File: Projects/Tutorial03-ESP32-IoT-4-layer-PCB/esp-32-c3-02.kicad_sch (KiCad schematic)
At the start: 30 parts, among them J3 GSD090012SEU, U3 ESP32-C3-WROOM-02-H4, U4 CP2102N-Axx-xQFN20, U5 USBLC6-2SC6, U6 W25Q32JVSSIQ

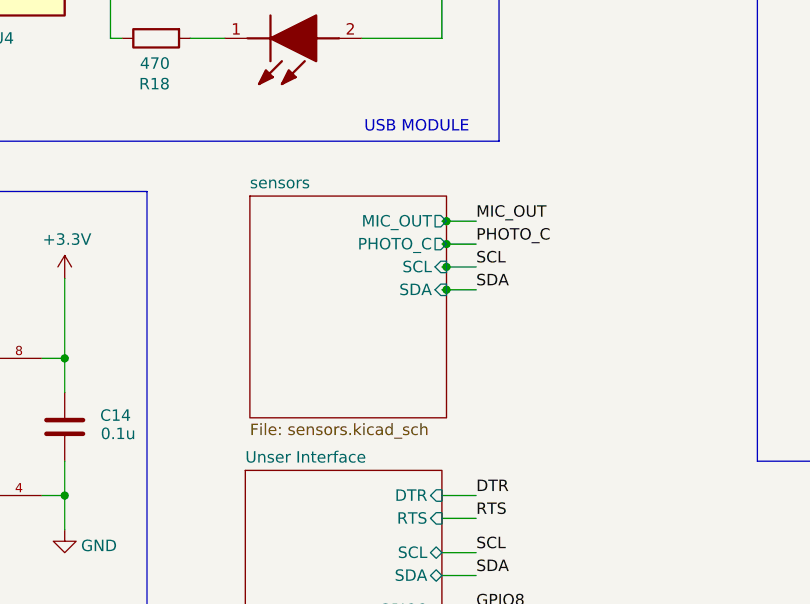
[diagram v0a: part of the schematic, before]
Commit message: 20260501
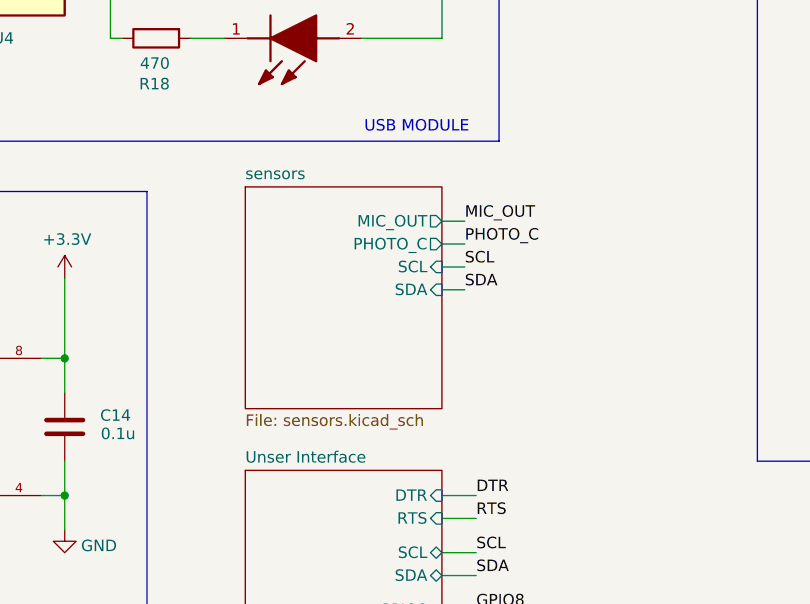
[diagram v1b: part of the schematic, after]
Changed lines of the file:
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@@
 	)
 	(junction
-		(at 141.478 134.62)
-		(diameter 0)
-		(color 0 0 0 0)
-	)
-	(junction
 		(at 59.69 35.56)
 		(diameter 0)
@@
 	)
 	(junction
-		(at 141.478 142.24)
-		(diameter 0)
-		(color 0 0 0 0)
-	)
-	(junction
 		(at 271.78 52.07)
 		(diameter 0)
@@
 	)
 	(junction
-		(at 141.478 137.16)
-		(diameter 0)
-		(color 0 0 0 0)
-	)
-	(junction
 		(at 242.57 45.72)
 		(diameter 0)
@@
 		(color 0 0 0 0)
 	)
-	(junction
-		(at 141.478 139.7)
-		(diameter 0)
-		(color 0 0 0 0)
-	)
 	(no_connect
 		(at 101.6 78.74)
@@
 	(wire
 		(pts
-			(xy 140.97 137.16) (xy 141.478 137.16)
-		)
-		(stroke
-			(width 0)
-			(type default)
-		)
-	)
-	(wire
-		(pts
 			(xy 22.86 76.2) (xy 35.56 76.2)
 		)
@@
 	(wire
 		(pts
-			(xy 141.478 139.7) (xy 144.78 139.7)
+			(xy 140.97 142.24) (xy 143.51 142.24)
 		)
 		(stroke
@@
 	(wire
 		(pts
-			(xy 141.478 142.24) (xy 144.78 142.24)
+			(xy 256.54 59.69) (xy 259.08 59.69)
 		)
 		(stroke
@@
 	(wire
 		(pts
-			(xy 256.54 59.69) (xy 259.08 59.69)
+			(xy 35.56 91.44) (xy 22.86 91.44)
 		)
 		(stroke
@@
 	(wire
 		(pts
-			(xy 35.56 91.44) (xy 22.86 91.44)
+			(xy 242.57 85.09) (xy 238.76 85.09)
 		)
 		(stroke
@@
 	(wire
 		(pts
-			(xy 242.57 85.09) (xy 238.76 85.09)
+			(xy 193.04 74.93) (xy 203.2 74.93)
 		)
 		(stroke
@@
 	(wire
 		(pts
-			(xy 193.04 74.93) (xy 203.2 74.93)
+			(xy 140.97 134.62) (xy 143.51 134.62)
 		)
 		(stroke
@@
 	(wire
 		(pts
-			(xy 140.97 134.62) (xy 141.478 134.62)
-		)
-		(stroke
-			(width 0)
-			(type default)
-		)
-	)
-	(wire
-		(pts
 			(xy 228.6 149.86) (xy 232.41 149.86)
 		)
@@
 	(wire
 		(pts
-			(xy 141.478 134.62) (xy 144.78 134.62)
-		)
-		(stroke
-			(width 0)
-			(type default)
-		)
-	)
-	(wire
-		(pts
 			(xy 22.86 91.44) (xy 22.86 95.25)
 		)
@@
 	(wire
 		(pts
-			(xy 140.97 139.7) (xy 141.478 139.7)
-		)
-		(stroke
-			(width 0)
-			(type default)
-		)
-	)
-	(wire
-		(pts
 			(xy 99.06 161.29) (xy 99.06 165.1)
 		)
@@
 	(wire
 		(pts
-			(xy 140.97 142.24) (xy 141.478 142.24)
-		)
-		(stroke
-			(width 0)
-			(type default)
-		)
-	)
-	(wire
-		(pts
 			(xy 99.06 165.1) (xy 99.06 168.91)
 		)
@@
 	(wire
 		(pts
+			(xy 140.97 139.7) (xy 143.51 139.7)
+		)
+		(stroke
+			(width 0)
+			(type default)
+		)
+	)
+	(wire
+		(pts
 			(xy 104.14 101.6) (xy 104.14 114.3)
 		)
@@
 	(wire
 		(pts
-			(xy 161.29 41.91) (xy 163.83 41.91)
+			(xy 140.97 137.16) (xy 143.51 137.16)
 		)
 		(stroke
@@
 	(wire
 		(pts
-			(xy 248.92 118.11) (xy 262.89 118.11)
+			(xy 161.29 41.91) (xy 163.83 41.91)
 		)
 		(stroke
@@
 	(wire
 		(pts
-			(xy 256.54 45.72) (xy 271.78 45.72)
+			(xy 248.92 118.11) (xy 262.89 118.11)
 		)
 		(stroke
@@
 	(wire
 		(pts
-			(xy 88.9 58.42) (xy 88.9 50.8)
+			(xy 256.54 45.72) (xy 271.78 45.72)
 		)
 		(stroke
@@
 	(wire
 		(pts
-			(xy 101.6 68.58) (xy 104.14 68.58)
+			(xy 88.9 58.42) (xy 88.9 50.8)
 		)
 		(stroke
@@
 	(wire
 		(pts
-			(xy 200.66 64.77) (xy 203.2 64.77)
+			(xy 101.6 68.58) (xy 104.14 68.58)
 		)
 		(stroke
@@
 	(wire
 		(pts
-			(xy 262.89 124.46) (xy 262.89 132.08)
+			(xy 200.66 64.77) (xy 203.2 64.77)
 		)
 		(stroke
@@
 	(wire
 		(pts
-			(xy 141.478 137.16) (xy 144.78 137.16)
+			(xy 262.89 124.46) (xy 262.89 132.08)
 		)
 		(stroke
@@
 	)
 	(label "SCL"
-		(at 144.78 139.7 0)
+		(at 143.51 139.7 0)
 		(effects
 			(font
@@
 	)
 	(label "SDA"
-		(at 144.78 142.24 0)
+		(at 143.51 142.24 0)
 		(effects
 			(font
@@
 	)
 	(label "MIC_OUT"
-		(at 144.78 134.62 0)
+		(at 143.51 134.62 0)
 		(effects
 			(font
@@
 	)
 	(label "PHOTO_C"
-		(at 144.78 137.16 0)
+		(at 143.51 137.16 0)
 		(effects
 			(font
@@
 	)
 	(sheet
-		(at 119.634 131.826)
+		(at 119.126 130.81)
 		(size 21.844 24.638)
 		(exclude_from_sim no)
@@
 		)
 		(property "Sheetname" "sensors"
-			(at 119.634 131.1144 0)
+			(at 119.126 130.0984 0)
 			(effects
 				(font
@@
 		)
 		(property "Sheetfile" "sensors.kicad_sch"
-			(at 119.634 157.0486 0)
+			(at 119.126 156.0326 0)
 			(effects
 				(font
@@
 		)
 		(pin "MIC_OUT" output
-			(at 141.478 134.62 0)
+			(at 140.97 134.62 0)
 			(effects
 				(font
@@
 		)
 		(pin "PHOTO_C" output
-			(at 141.478 137.16 0)
+			(at 140.97 137.16 0)
 			(effects
 				(font
@@
 		)
 		(pin "SCL" input
-			(at 141.478 139.7 0)
+			(at 140.97 139.7 0)
 			(effects
 				(font
@@
 		)
 		(pin "SDA" input
-			(at 141.478 142.24 0)
+			(at 140.97 142.24 0)
 			(effects
 				(font

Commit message: 20260516
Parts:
- U4: footprint Package_DFN_QFN:SiliconLabs_QFN-20-1EP_3x3mm_P0.5mm -> ESP32 Project Footprints:QFN20P400X400X100-21N
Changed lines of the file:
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@@
 			)
 		)
-		(property "Footprint" "Package_DFN_QFN:SiliconLabs_QFN-20-1EP_3x3mm_P0.5mm"
+		(property "Footprint" "ESP32 Project Footprints:QFN20P400X400X100-21N"
 			(at 120.65 113.03 0)
 			(effects

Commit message: 20260525
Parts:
- C12, C7, C9: footprint ESP32 Project Footprints:T491A -> Project-Footprints:T491A
- J3: footprint ESP32 Project Footprints:AMPHENOL_GSD090012SEU -> Project-Footprints:AMPHENOL_GSD090012SEU
- LED5-GREEN1: footprint ESP32 Project Footprints:LEDC2012X120N -> Project-Footprints:T491A
- LED6-RED1: footprint ESP32 Project Footprints:LEDC2012X120N -> Project-Footprints:LEDC2012X120N
- U3: footprint ESP32-C3-WROOM-02-H4:MODULE_ESP32-C3-WROOM-02-H4 -> Project-Footprints:MODULE_ESP32-C3-WROOM-02-H4
- U4: footprint ESP32 Project Footprints:QFN20P400X400X100-21N -> Project-Footprints:QFN20P400X400X100-21N
- U6: footprint W25Q32JVSSIQ:SOIC127P790X216-8N -> Package_SON:WSON-8-1EP_6x5mm_P1.27mm_EP3.4x4.3mm
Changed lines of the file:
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@@
 			)
 		)
-		(property "Footprint" "W25Q32JVSSIQ:SOIC127P790X216-8N"
+		(property "Footprint" "Package_SON:WSON-8-1EP_6x5mm_P1.27mm_EP3.4x4.3mm"
 			(at 78.74 157.48 0)
 			(effects
@@
 			)
 		)
-		(property "Footprint" "ESP32 Project Footprints:T491A"
+		(property "Footprint" "Project-Footprints:T491A"
 			(at 256.54 44.7548 0)
 			(effects
@@
 			)
 		)
-		(property "Footprint" "ESP32 Project Footprints:LEDC2012X120N"
+		(property "Footprint" "Project-Footprints:LEDC2012X120N"
 			(at 129.54 20.65 0)
 			(effects
@@
 			)
 		)
-		(property "Footprint" "ESP32 Project Footprints:T491A"
+		(property "Footprint" "Project-Footprints:T491A"
 			(at 241.3 117.1448 0)
 			(effects
@@
 			)
 		)
-		(property "Footprint" "ESP32 Project Footprints:T491A"
+		(property "Footprint" "Project-Footprints:T491A"
 			(at 72.39 34.5948 0)
 			(effects
@@
 			)
 		)
-		(property "Footprint" "ESP32 Project Footprints:LEDC2012X120N"
+		(property "Footprint" "Project-Footprints:T491A"
 			(at 129.54 5.41 0)
 			(effects
@@
 			)
 		)
-		(property "Footprint" "ESP32-C3-WROOM-02-H4:MODULE_ESP32-C3-WROOM-02-H4"
+		(property "Footprint" "Project-Footprints:MODULE_ESP32-C3-WROOM-02-H4"
 			(at 220.98 69.85 0)
 			(effects
@@
 			)
 		)
-		(property "Footprint" "ESP32 Project Footprints:QFN20P400X400X100-21N"
+		(property "Footprint" "Project-Footprints:QFN20P400X400X100-21N"
 			(at 120.65 113.03 0)
 			(effects
@@
 			)
 		)
-		(property "Footprint" "ESP32 Project Footprints:AMPHENOL_GSD090012SEU"
+		(property "Footprint" "Project-Footprints:AMPHENOL_GSD090012SEU"
 			(at 210.82 137.16 0)
 			(effects
